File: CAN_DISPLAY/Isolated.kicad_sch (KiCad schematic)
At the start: 38 parts, among them J20 NMEA0183, J4 NMEA2000, J8 DCDC 5V, U3 ISO1050DUB, U4 AMS1117-5.0, U5 ISO3080DW

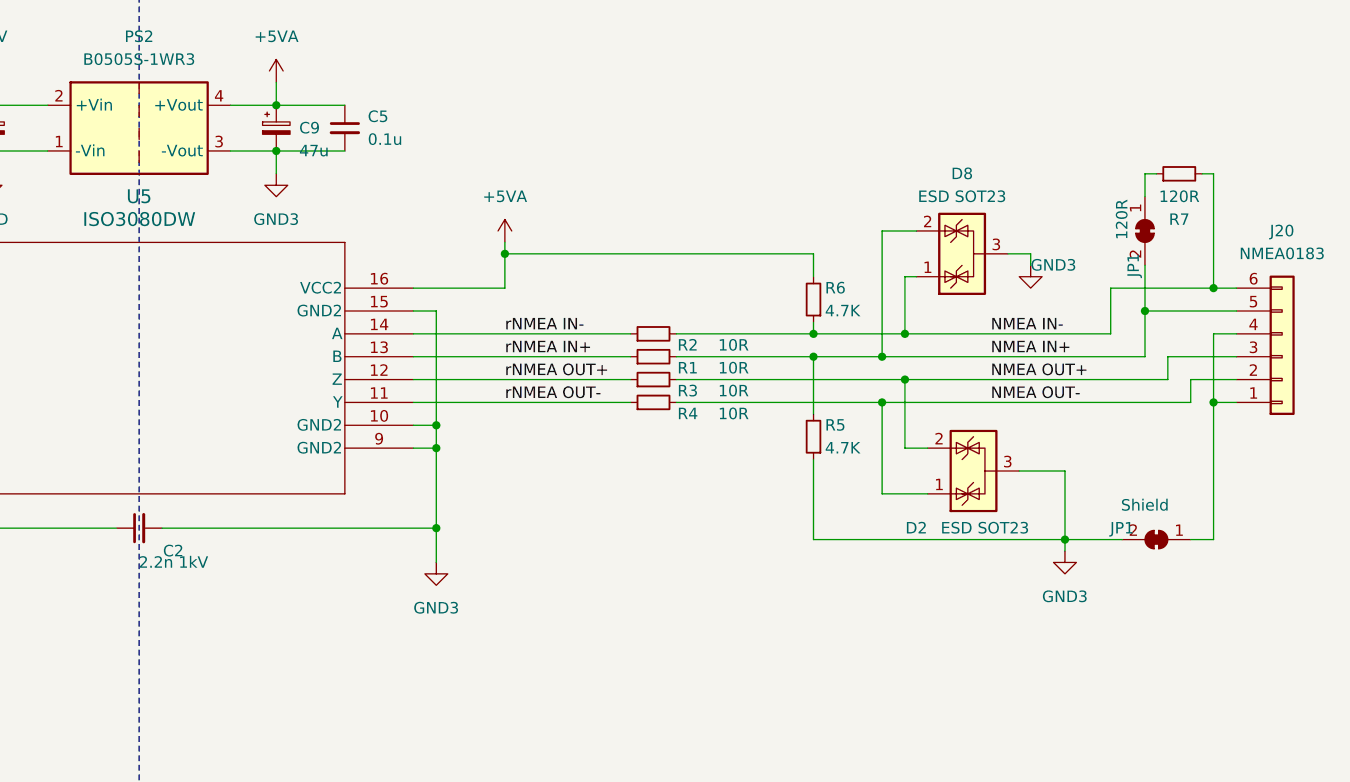
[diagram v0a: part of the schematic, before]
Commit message: 1234
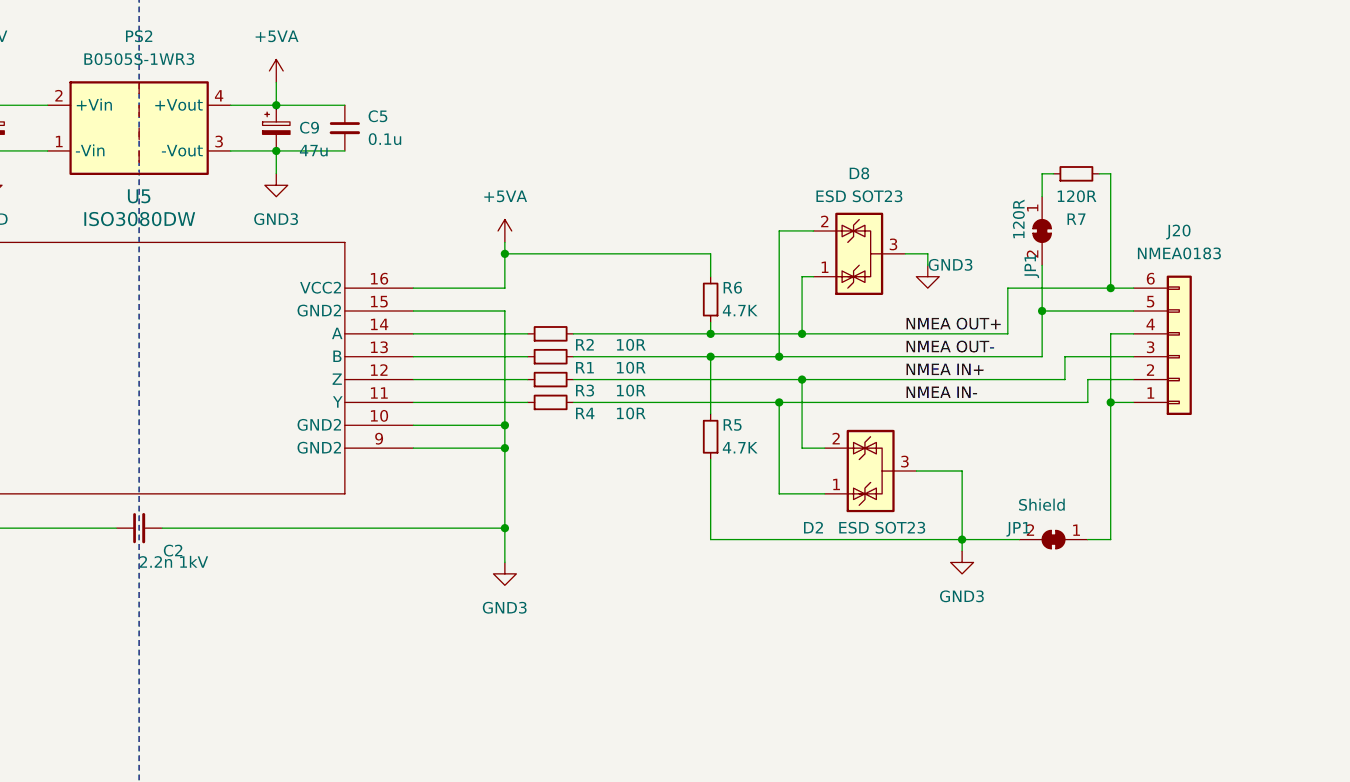
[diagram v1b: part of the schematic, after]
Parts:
- J20: footprint TerminalBlock:TerminalBlock_bornier-6_P5.08mm -> TerminalBlock_Altech:Altech_AK300_1x06_P5.00mm_45-Degree
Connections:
- net NMEA IN+: now also D2.2 (K), J20.3 (Pin_3), R3.2; no longer D8.2 (K), J20.5 (Pin_5), JP1.2 (B), R1.2, R5.2
- net NMEA IN-: now also D2.1 (K), J20.2 (Pin_2), R4.2; no longer D8.1 (K), J20.6 (Pin_6), R2.2, R6.1, R7.2
- net NMEA OUT+: now also D8.1 (K), J20.6 (Pin_6), R2.2, R6.1, R7.2; no longer D2.2 (K), J20.3 (Pin_3), R3.2
- net NMEA OUT-: now also D8.2 (K), J20.5 (Pin_5), JP1.2 (B), R1.2, R5.2; no longer D2.1 (K), J20.2 (Pin_2), R4.2
- net rNMEA IN+: no longer names the net of R1.1, U5.13 (B)
- net rNMEA IN-: no longer names the net of R2.1, U5.14 (A)
- net rNMEA OUT+: no longer names the net of R3.1, U5.12 (Z)
- net rNMEA OUT-: no longer names the net of R4.1, U5.11 (Y)
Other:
- moved on the sheet: D2, D8, J20, JP1, R1, R2, R3, R4, R5, R6, R7
